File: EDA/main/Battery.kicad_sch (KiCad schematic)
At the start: 84 parts, among them J5 STM32L0_SWD, J7 SKRPACE010, J8 Power, J9 XT30 Battery, U1 TPS63060DSCT, U10 TPS25730DREFR, U11 STM32L031G6U6, U14 TPS63060DSCT, U9 BQ25895RTWT, Y1 ABS07-32.768KHZ-T

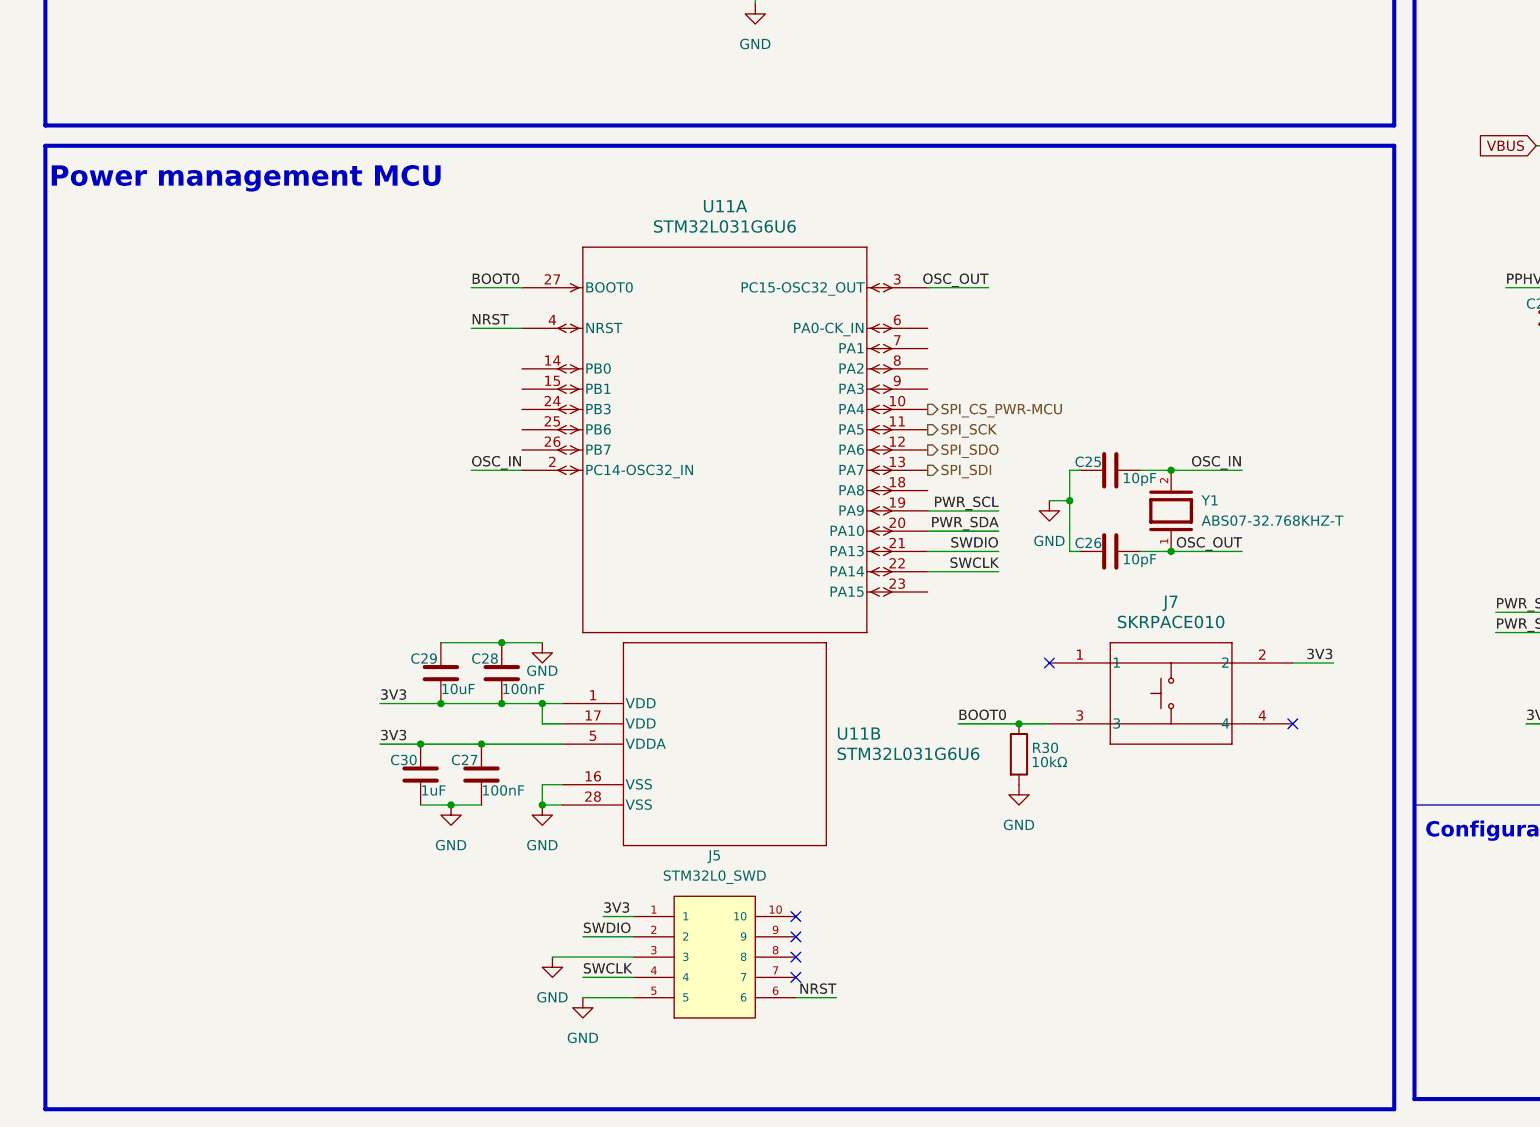
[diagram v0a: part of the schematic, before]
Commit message: Uploaded work
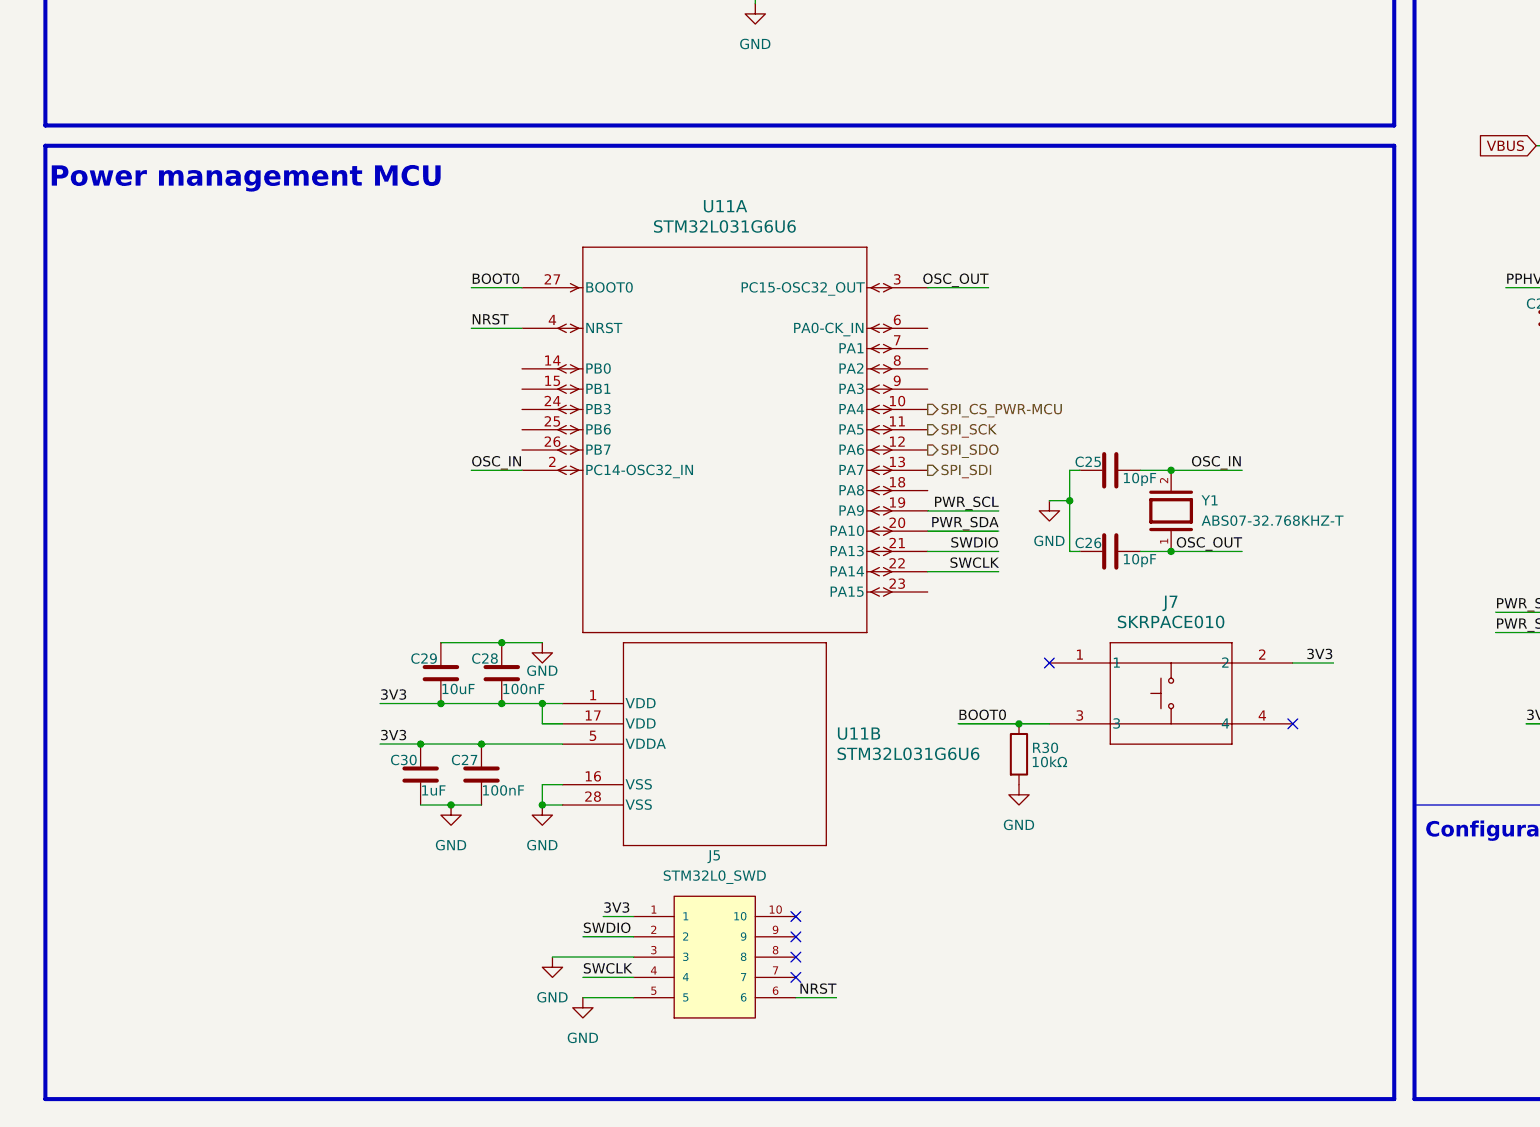
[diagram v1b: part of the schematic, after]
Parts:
- L1, L3: footprint (none) -> Inductor_SMD:L_1008_2520Metric; Manufacturer Part (none) -> 74438324010
- L2: footprint (none) -> Inductor_SMD:L_Wuerth_MAPI-4020; Manufacturer Part (none) -> 74438356022
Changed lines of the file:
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@@
 	(rectangle
 		(start 64.77 130.81)
-		(end 233.68 251.46)
+		(end 233.68 250.19)
 		(stroke
 			(width 0.508)
@@
 			)
 		)
-		(property "Footprint" ""
+		(property "Footprint" "Inductor_SMD:L_Wuerth_MAPI-4020"
 			(at 186.69 54.61 0)
 			(effects
@@
 			)
 		)
+		(property "Manufacturer Part" "74438356022"
+			(at 186.69 54.61 90)
+			(effects
+				(font
+					(size 1.27 1.27)
+				)
+				(hide yes)
+			)
+		)
 		(pin "1"
 		)
@@
 			)
 		)
-		(property "Footprint" ""
+		(property "Footprint" "Inductor_SMD:L_1008_2520Metric"
 			(at 289.56 68.58 0)
 			(effects
@@
 			)
 		)
+		(property "Manufacturer Part" "74438324010"
+			(at 289.56 68.58 0)
+			(effects
+				(font
+					(size 1.27 1.27)
+				)
+				(hide yes)
+			)
+		)
 		(pin "1"
 		)
@@
 			)
 		)
-		(property "Footprint" ""
+		(property "Footprint" "Inductor_SMD:L_1008_2520Metric"
 			(at 461.01 68.58 0)
 			(effects
@@
 			(at 461.01 68.58 0)
 			(effects
+				(font
+					(size 1.27 1.27)
+				)
+				(hide yes)
+			)
+		)
+		(property "Manufacturer Part" "74438324010"
+			(at 461.01 68.58 0)
+			(effects
